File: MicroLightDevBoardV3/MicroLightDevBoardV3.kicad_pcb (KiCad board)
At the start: 4 copper layers, 12.9 x 18.9 mm, 30 parts, among them J1 TYPE-C-31-M-12, J2 Conn_01x02_Socket, J3 Conn_01x03_Socket, J4 Conn_01x01_Socket, J5 Conn_01x01_Socket, SW1 SW_Push, U1 USBLC6-2P6, U2 STM32C071GBUx, U3 BQ25180, U4 S-85S1AB33-I6T1U, U7 MC3479

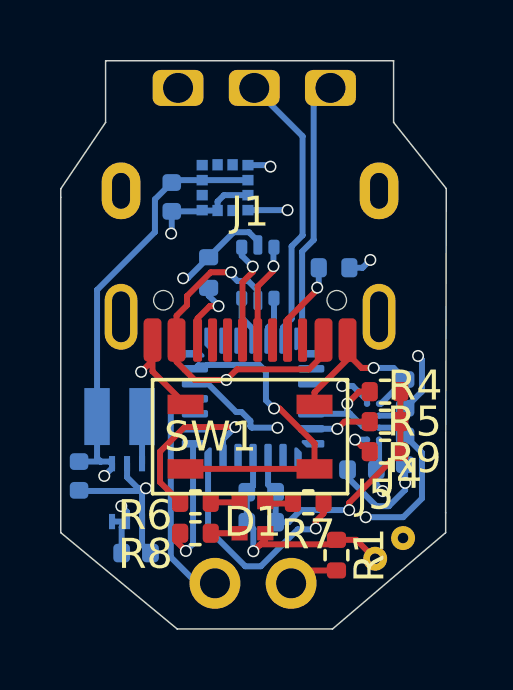
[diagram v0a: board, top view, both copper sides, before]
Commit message: cleanup
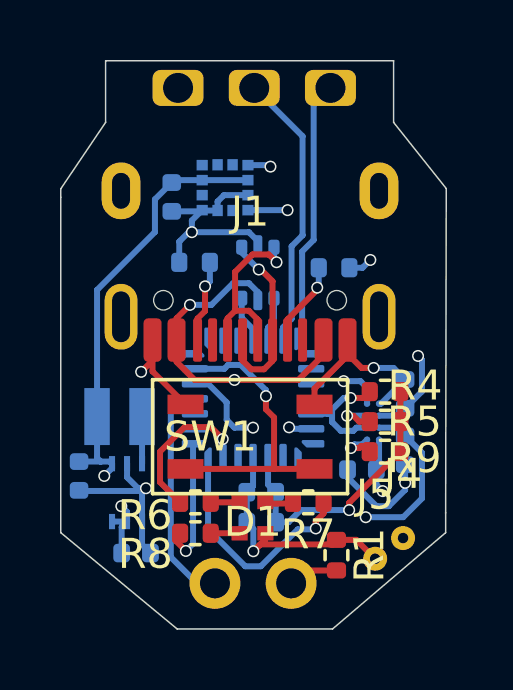
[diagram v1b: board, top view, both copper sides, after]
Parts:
- moved R3 0.58 mm to (34.9, 24.0), turned to 180 degrees
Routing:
- net Net-(J1-D+-PadA6): track 3.32 -> 6.20 mm
- net Net-(J1-D--PadA7): track 3.39 -> 6.18 mm
- net I2C_SDA: track 14.5 -> 16.3 mm, vias 2 -> 3
- net red: track 5.98 -> 5.16 mm
- net INT_CHRG: track 7.39 -> 8.13 mm
- net GND: track 43.5 -> 43.9 mm, vias 8 -> 7
